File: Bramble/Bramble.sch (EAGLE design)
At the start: 10 parts

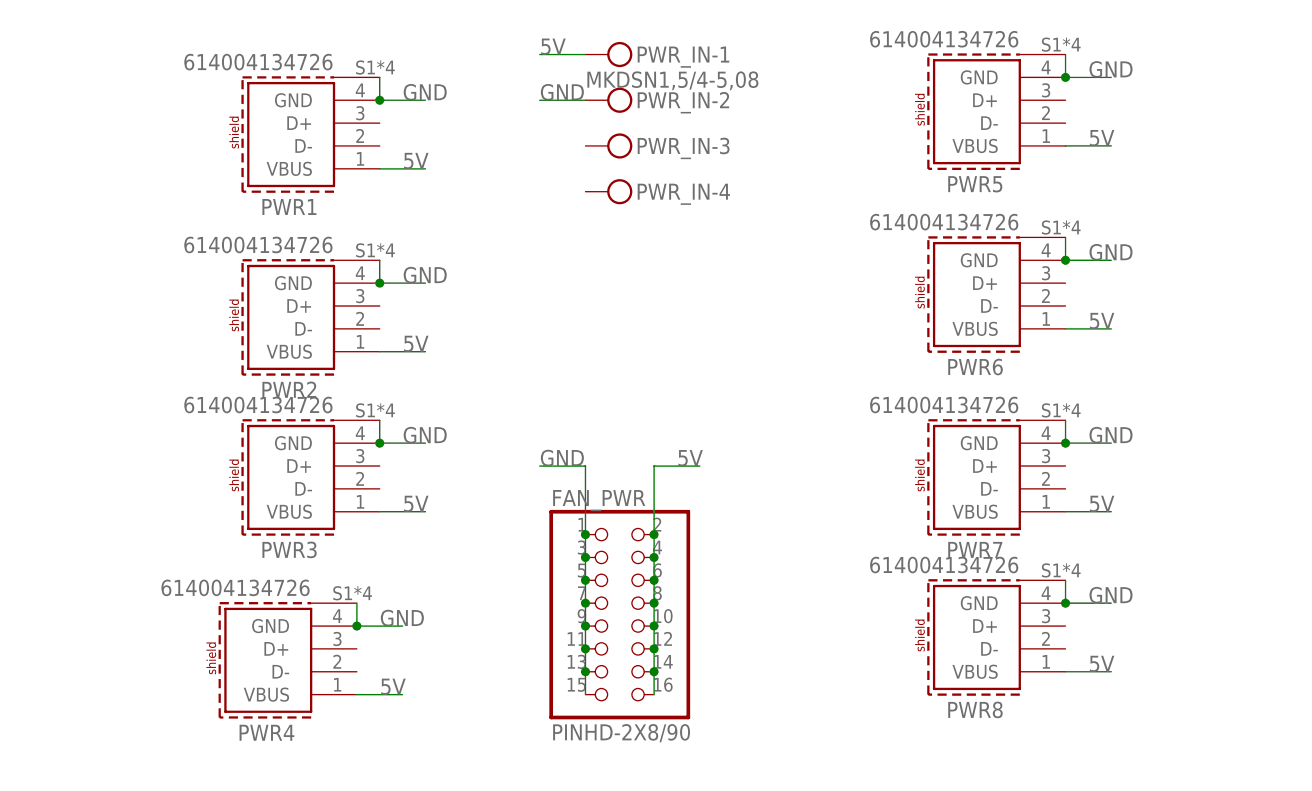
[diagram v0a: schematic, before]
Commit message: Upgrades
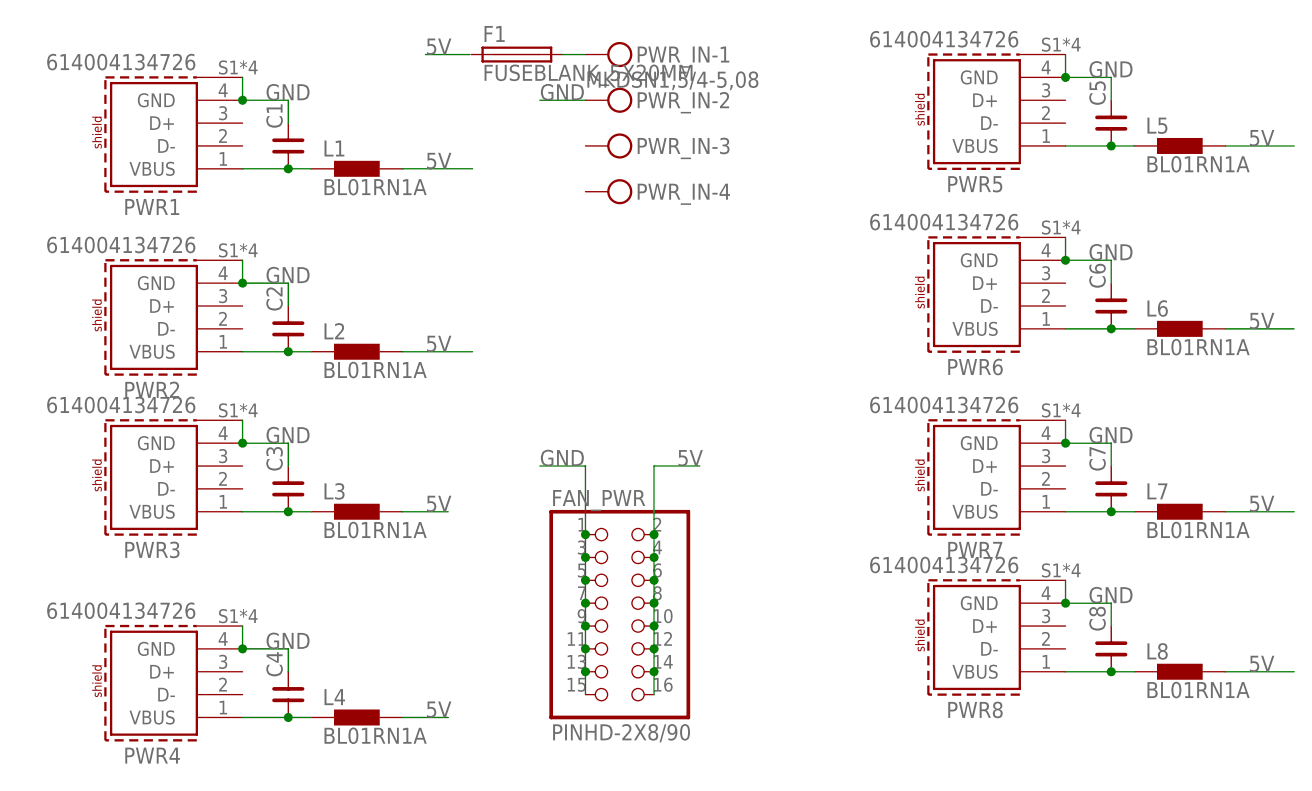
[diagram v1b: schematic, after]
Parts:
- added C1, C2, C3, C4, C5, C6, C7, C8: (no value), cap-master:CBP-ENP-020-050
- added F1: FUSEBLANK_5X20MM, fuse:FUSEBLANK_5X20MM
- added L1, L2, L3, L4, L5, L6, L7, L8: BL01RN1A, inductors:BL01RN1A
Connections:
- new net N$1: C1.1, L1.1, PWR1.VBUS
- new net N$2: C2.1, L2.1, PWR2.VBUS
- new net N$3: C4.1, L4.1, PWR4.VBUS
- new net N$4: C3.1, L3.1, PWR3.VBUS
- new net N$5: C5.1, L5.1, PWR5.VBUS
- new net N$6: C6.1, L6.1, PWR6.VBUS
- new net N$7: C7.1, L7.1, PWR7.VBUS
- new net N$8: C8.1, L8.1, PWR8.VBUS
- new net N$9: F1.2, PWR_IN-1.KL
- net 5V: now also L1.2, L2.2, L3.2, L4.2, L5.2, L6.2, L7.2, L8.2; no longer PWR1.VBUS, PWR2.VBUS, PWR3.VBUS, PWR4.VBUS, PWR5.VBUS, PWR6.VBUS, PWR7.VBUS, PWR8.VBUS, PWR_IN-1.KL
- net GND: now also C1.2, C2.2, C3.2, C4.2, C5.2, C6.2, C7.2, C8.2
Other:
- moved on the sheet: PWR1, PWR2, PWR3, PWR4
